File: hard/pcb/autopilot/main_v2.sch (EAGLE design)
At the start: 169 parts, among them IC1 24AA32ASN, IC2 INA194, IC3 LP2950Z, Q1 IRLML5203, Q3 IRLML5203, Q4 IRLML5203, T3 BC848, U2 TMP75DGK, U44 BMP085, X1 USB-SMD-NS

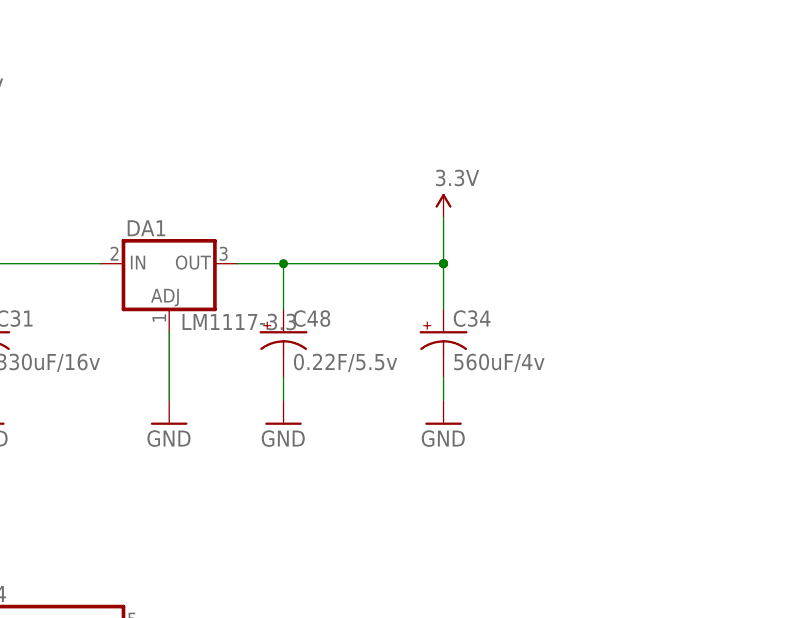
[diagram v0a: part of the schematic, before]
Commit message: Added board v2
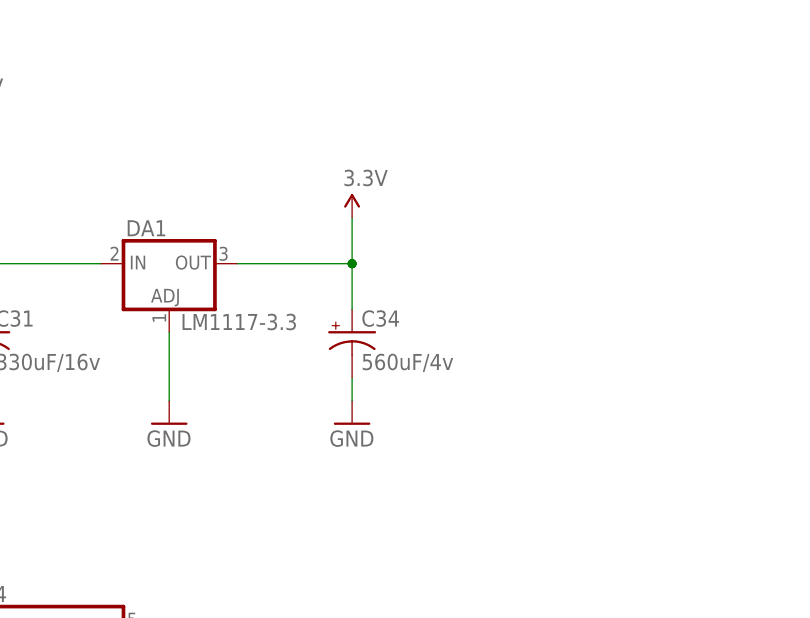
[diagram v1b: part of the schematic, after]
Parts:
- removed C48: 0.22F/5.5v, barthess:CAP_POLIONISTOR
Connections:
- net 3.3V: no longer C48.+
- net GND: no longer C48.-
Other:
- moved on the sheet: C34
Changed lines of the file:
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@@
 <setting verticaltext="up"/>
 </settings>
-<grid distance="0.1" unitdist="inch" unit="inch" style="lines" multiple="1" display="yes" altdistance="0.01" altunitdist="inch" altunit="inch"/>
+<grid distance="0.1" unitdist="inch" unit="inch" style="lines" multiple="1" display="no" altdistance="0.01" altunitdist="inch" altunit="inch"/>
 <layers>
-<layer number="1" name="Top" color="4" fill="1" visible="no" active="no"/>
-<layer number="16" name="Bottom" color="1" fill="1" visible="no" active="no"/>
-<layer number="17" name="Pads" color="2" fill="1" visible="no" active="no"/>
-<layer number="18" name="Vias" color="2" fill="1" visible="no" active="no"/>
-<layer number="19" name="Unrouted" color="6" fill="1" visible="no" active="no"/>
-<layer number="20" name="Dimension" color="15" fill="1" visible="no" active="no"/>
-<layer number="21" name="tPlace" color="7" fill="1" visible="no" active="no"/>
-<layer number="22" name="bPlace" color="7" fill="1" visible="no" active="no"/>
-<layer number="23" name="tOrigins" color="15" fill="1" visible="no" active="no"/>
-<layer number="24" name="bOrigins" color="15" fill="1" visible="no" active="no"/>
-<layer number="25" name="tNames" color="7" fill="1" visible="no" active="no"/>
-<layer number="26" name="bNames" color="7" fill="1" visible="no" active="no"/>
-<layer number="27" name="tValues" color="7" fill="1" visible="no" active="no"/>
-<layer number="28" name="bValues" color="7" fill="1" visible="no" active="no"/>
+<layer number="1" name="Top" color="4" fill="1" visible="yes" active="no"/>
+<layer number="16" name="Bottom" color="1" fill="1" visible="yes" active="no"/>
+<layer number="17" name="Pads" color="2" fill="1" visible="yes" active="no"/>
+<layer number="18" name="Vias" color="2" fill="1" visible="yes" active="no"/>
+<layer number="19" name="Unrouted" color="6" fill="1" visible="yes" active="no"/>
+<layer number="20" name="Dimension" color="15" fill="1" visible="yes" active="no"/>
+<layer number="21" name="tPlace" color="7" fill="1" visible="yes" active="no"/>
+<layer number="22" name="bPlace" color="7" fill="1" visible="yes" active="no"/>
+<layer number="23" name="tOrigins" color="15" fill="1" visible="yes" active="no"/>
+<layer number="24" name="bOrigins" color="15" fill="1" visible="yes" active="no"/>
+<layer number="25" name="tNames" color="7" fill="1" visible="yes" active="no"/>
+<layer number="26" name="bNames" color="7" fill="1" visible="yes" active="no"/>
+<layer number="27" name="tValues" color="7" fill="1" visible="yes" active="no"/>
+<layer number="28" name="bValues" color="7" fill="1" visible="yes" active="no"/>
 <layer number="29" name="tStop" color="7" fill="3" visible="no" active="no"/>
 <layer number="30" name="bStop" color="7" fill="6" visible="no" active="no"/>
@@
 <layer number="35" name="tGlue" color="7" fill="4" visible="no" active="no"/>
 <layer number="36" name="bGlue" color="7" fill="5" visible="no" active="no"/>
-<layer number="37" name="tTest" color="7" fill="1" visible="no" active="no"/>
-<layer number="38" name="bTest" color="7" fill="1" visible="no" active="no"/>
+<layer number="37" name="tTest" color="7" fill="1" visible="yes" active="no"/>
+<layer number="38" name="bTest" color="7" fill="1" visible="yes" active="no"/>
 <layer number="39" name="tKeepout" color="4" fill="11" visible="no" active="no"/>
 <layer number="40" name="bKeepout" color="1" fill="11" visible="no" active="no"/>
@@
 <layer number="44" name="Drills" color="7" fill="1" visible="no" active="no"/>
 <layer number="45" name="Holes" color="7" fill="1" visible="no" active="no"/>
-<layer number="46" name="Milling" color="3" fill="1" visible="no" active="no"/>
-<layer number="47" name="Measures" color="7" fill="1" visible="no" active="no"/>
-<layer number="48" name="Document" color="7" fill="1" visible="no" active="no"/>
-<layer number="49" name="Reference" color="7" fill="1" visible="no" active="no"/>
-<layer number="50" name="dxf" color="7" fill="1" visible="no" active="no"/>
-<layer number="51" name="tDocu" color="14" fill="1" visible="no" active="no"/>
-<layer number="52" name="bDocu" color="7" fill="1" visible="no" active="no"/>
-<layer number="53" name="tGND_GNDA" color="7" fill="9" visible="no" active="no"/>
-<layer number="54" name="bGND_GNDA" color="1" fill="9" visible="no" active="no"/>
-<layer number="56" name="wert" color="7" fill="1" visible="no" active="no"/>
+<layer number="46" name="Milling" color="3" fill="1" visible="yes" active="no"/>
+<layer number="47" name="Measures" color="7" fill="1" visible="yes" active="no"/>
+<layer number="48" name="Document" color="7" fill="1" visible="yes" active="no"/>
+<layer number="49" name="Reference" color="7" fill="1" visible="yes" active="no"/>
+<layer number="50" name="dxf" color="7" fill="1" visible="yes" active="no"/>
+<layer number="51" name="tDocu" color="7" fill="1" visible="yes" active="no"/>
+<layer number="52" name="bDocu" color="7" fill="1" visible="yes" active="no"/>
+<layer number="53" name="tGND_GNDA" color="7" fill="9" visible="yes" active="no"/>
+<layer number="54" name="bGND_GNDA" color="1" fill="9" visible="yes" active="no"/>
+<layer number="56" name="wert" color="7" fill="1" visible="yes" active="no"/>
 <layer number="91" name="Nets" color="2" fill="1" visible="yes" active="yes"/>
 <layer number="92" name="Busses" color="1" fill="1" visible="yes" active="yes"/>
@@
 <part name="R32" library="SparkFun" deviceset="RESISTOR" device="0805-RES" value="100k"/>
 <part name="XP6" library="SparkFun" deviceset="JUMPER-3" device="PTH" value="sonar"/>
-<part name="C48" library="barthess" deviceset="CAP_POL" device="IONISTOR" value="0.22F/5.5v"/>
-<part name="GND43" library="SparkFun" deviceset="GND" device=""/>
 <part name="XP8" library="SparkFun" deviceset="JUMPER-3" device="PTH" value="PWM1"/>
 <part name="XP9" library="SparkFun" deviceset="JUMPER-3" device="PTH" value="PWM2"/>
@@
 <instance part="GND28" gate="1" x="-248.92" y="-20.32"/>
 <instance part="GND30" gate="1" x="-269.24" y="-20.32"/>
-<instance part="P+18" gate="G$1" x="-218.44" y="2.54"/>
-<instance part="GND31" gate="1" x="-218.44" y="-20.32"/>
+<instance part="P+18" gate="G$1" x="-228.6" y="2.54"/>
+<instance part="GND31" gate="1" x="-228.6" y="-20.32"/>
 <instance part="R27" gate="G$1" x="119.38" y="68.58" rot="R90"/>
 <instance part="P+16" gate="G$1" x="109.22" y="76.2"/>
@@
 <instance part="R32" gate="G$1" x="63.5" y="-76.2" rot="R270"/>
 <instance part="XP6" gate="G$1" x="-154.94" y="-170.18" rot="MR270"/>
-<instance part="C48" gate="G$1" x="-236.22" y="-10.16"/>
-<instance part="GND43" gate="1" x="-236.22" y="-20.32"/>
 <instance part="XP8" gate="G$1" x="-101.6" y="-160.02"/>
 <instance part="XP9" gate="G$1" x="-88.9" y="-160.02"/>
@@
 <instance part="JP9" gate="G$1" x="-241.3" y="-170.18" rot="R90"/>
 <instance part="C31" gate="G$1" x="-269.24" y="-10.16"/>
-<instance part="C34" gate="G$1" x="-218.44" y="-10.16"/>
+<instance part="C34" gate="G$1" x="-228.6" y="-10.16"/>
 <instance part="XP16" gate="G$1" x="-154.94" y="-160.02" rot="R90"/>
 <instance part="GND10" gate="1" x="-129.54" y="-154.94" rot="R90"/>
@@
 </segment>
 <segment>
-<wire x1="-218.44" y1="-2.54" x2="-236.22" y2="-2.54" width="0.1524" layer="91"/>
-<wire x1="-236.22" y1="-2.54" x2="-241.3" y2="-2.54" width="0.1524" layer="91"/>
-<wire x1="-218.44" y1="-7.62" x2="-218.44" y2="-2.54" width="0.1524" layer="91"/>
-<wire x1="-218.44" y1="2.54" x2="-218.44" y2="-2.54" width="0.1524" layer="91"/>
-<wire x1="-236.22" y1="-7.62" x2="-236.22" y2="-2.54" width="0.1524" layer="91"/>
-<junction x="-218.44" y="-2.54"/>
-<junction x="-218.44" y="-2.54"/>
-<junction x="-236.22" y="-2.54"/>
+<wire x1="-228.6" y1="-2.54" x2="-241.3" y2="-2.54" width="0.1524" layer="91"/>
+<wire x1="-228.6" y1="-7.62" x2="-228.6" y2="-2.54" width="0.1524" layer="91"/>
+<wire x1="-228.6" y1="2.54" x2="-228.6" y2="-2.54" width="0.1524" layer="91"/>
+<junction x="-228.6" y="-2.54"/>
+<junction x="-228.6" y="-2.54"/>
 <pinref part="P+18" gate="G$1" pin="3.3V"/>
-<pinref part="C48" gate="G$1" pin="+"/>
 <pinref part="C34" gate="G$1" pin="+"/>
 <pinref part="DA1" gate="G$1" pin="OUT"/>
@@
 </segment>
 <segment>
-<wire x1="-218.44" y1="-17.78" x2="-218.44" y2="-15.24" width="0.1524" layer="91"/>
+<wire x1="-228.6" y1="-17.78" x2="-228.6" y2="-15.24" width="0.1524" layer="91"/>
 <pinref part="GND31" gate="1" pin="GND"/>
 <pinref part="C34" gate="G$1" pin="-"/>
@@
 </segment>
 <segment>
-<wire x1="-236.22" y1="-17.78" x2="-236.22" y2="-15.24" width="0.1524" layer="91"/>
-<pinref part="GND43" gate="1" pin="GND"/>
-<pinref part="C48" gate="G$1" pin="-"/>
-</segment>
-<segment>

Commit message: Changed in PCB
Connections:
- removed net N$12: C14.+, C15.1, DA4.EN, DA4.IN, L1.2
- new net N$30: C14.+, C15.1, DA4.EN, DA4.IN, L1.2, Q1.S, R59.1
- net 6V: no longer Q1.S, R59.1
- net I2C_FAST_SCL: now also DD1.PB6; no longer DD1.PB10
- net I2C_FAST_SDA: now also DD1.PB7; no longer DD1.PB11
- net I2C_SLOW_SCL: now also DD1.PB10; no longer DD1.PB6
- net I2C_SLOW_SDA: now also DD1.PB11; no longer DD1.PB7
- net MPXV_TEMP: now also DD1.PC2; no longer DD1.PC4
- net N$54: now also DD1.PC4; no longer DD1.PC2
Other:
- moved on the sheet: C14, C15, C16, C17, C18, C22, C43, C45, DA2, DA4, IC2, L1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
